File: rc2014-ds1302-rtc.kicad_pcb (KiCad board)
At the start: 2 copper layers, 100 x 50 mm, 16 parts, among them P1 RC2014 BUS, SW1 SW_DIP_x06, U1 74HCT688, U2 74LS125, U3 74LS174, U4 DS1302, U5 74LS32, Y1 Crystal

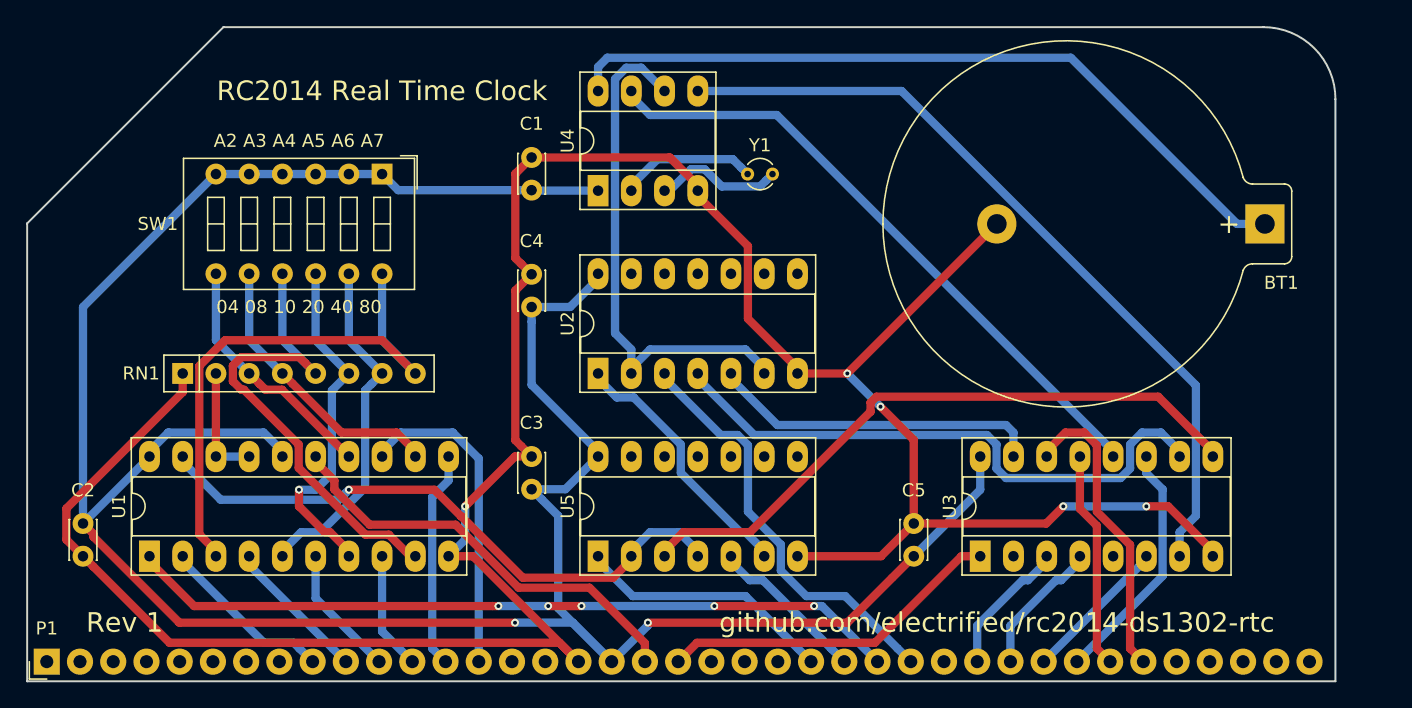
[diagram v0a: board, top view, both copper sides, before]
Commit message: after autoroute
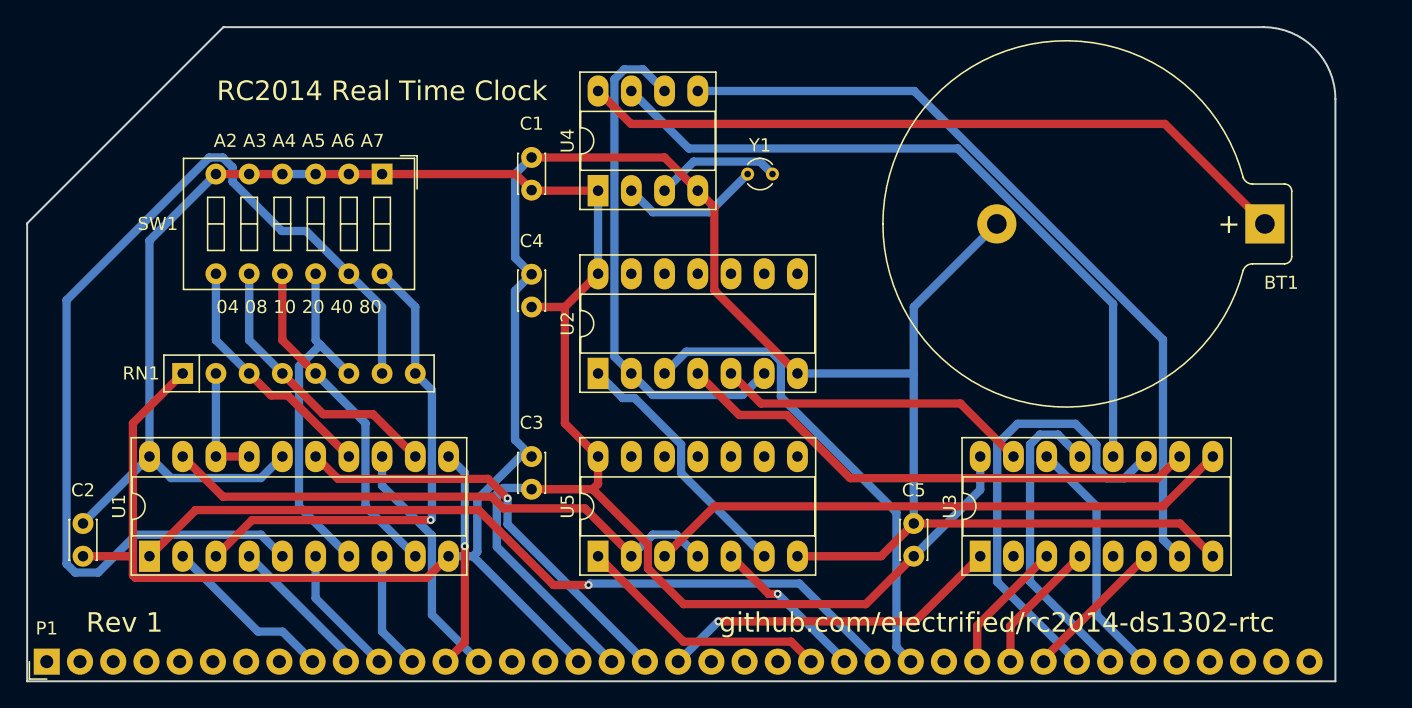
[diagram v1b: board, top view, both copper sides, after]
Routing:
- net Net-(RN1-Pad7): track 26.7 -> 77.9 mm
- net VCC: track 202.9 -> 164.3 mm, vias 2 -> 0
- net /D5: track 18.9 -> 34.7 mm
- net GND: track 208.4 -> 192.8 mm, vias 5 -> 0
- net Net-(RN1-Pad5): track 37.5 -> 25.8 mm
- net /D6: track 16.6 -> 24.0 mm
- net /RTC_CLK: track 48.9 -> 55.2 mm
- net /A2: track 24.7 -> 18.7 mm
- net //RTC_WR: track 49.7 -> 45.1 mm
- net /D0: track 32.3 -> 37.0 mm
- net /D7: track 23.2 -> 18.7 mm
- net /RTC_WE: track 45.0 -> 40.8 mm
- net Net-(RN1-Pad8): track 42.1 -> 38.0 mm, vias 0 -> 1
- net Net-(BT1-Pad1): track 58.4 -> 55.2 mm
- net //CS_RTC: track 46.9 -> 44.0 mm, vias 2 -> 0
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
